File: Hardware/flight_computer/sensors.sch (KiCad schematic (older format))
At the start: 21 parts

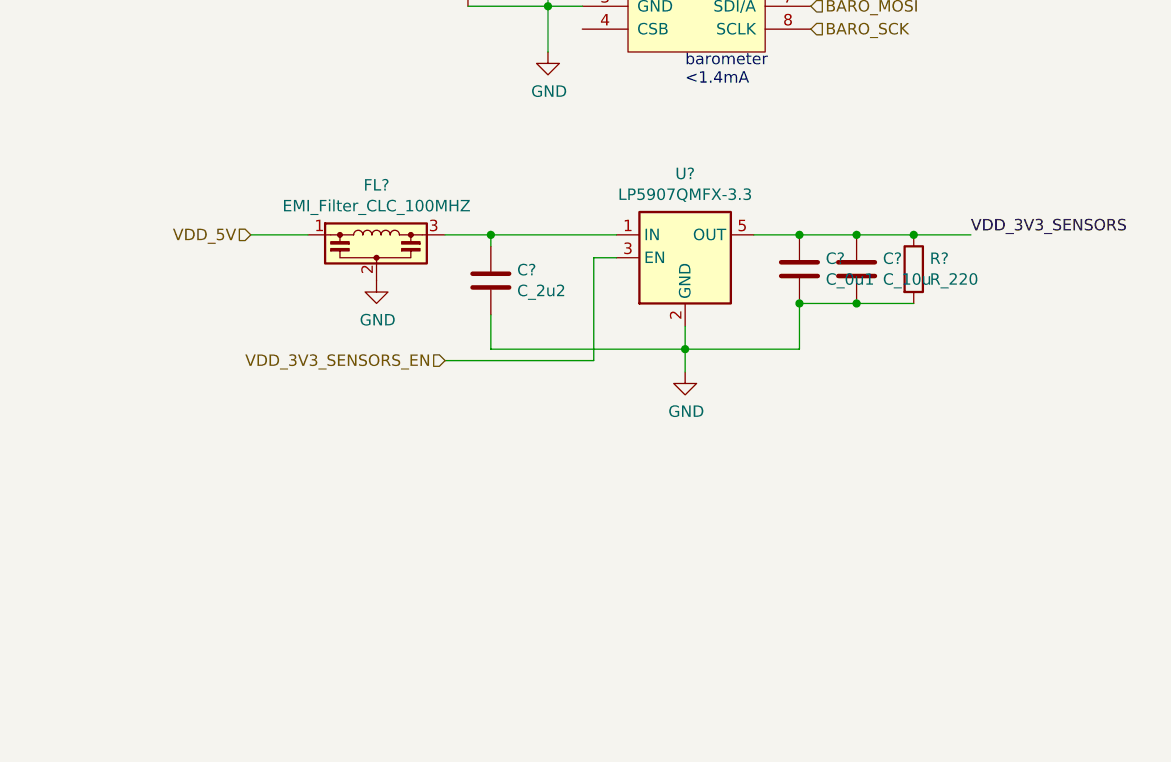
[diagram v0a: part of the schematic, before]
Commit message: added components, rerranged things to slow down dan
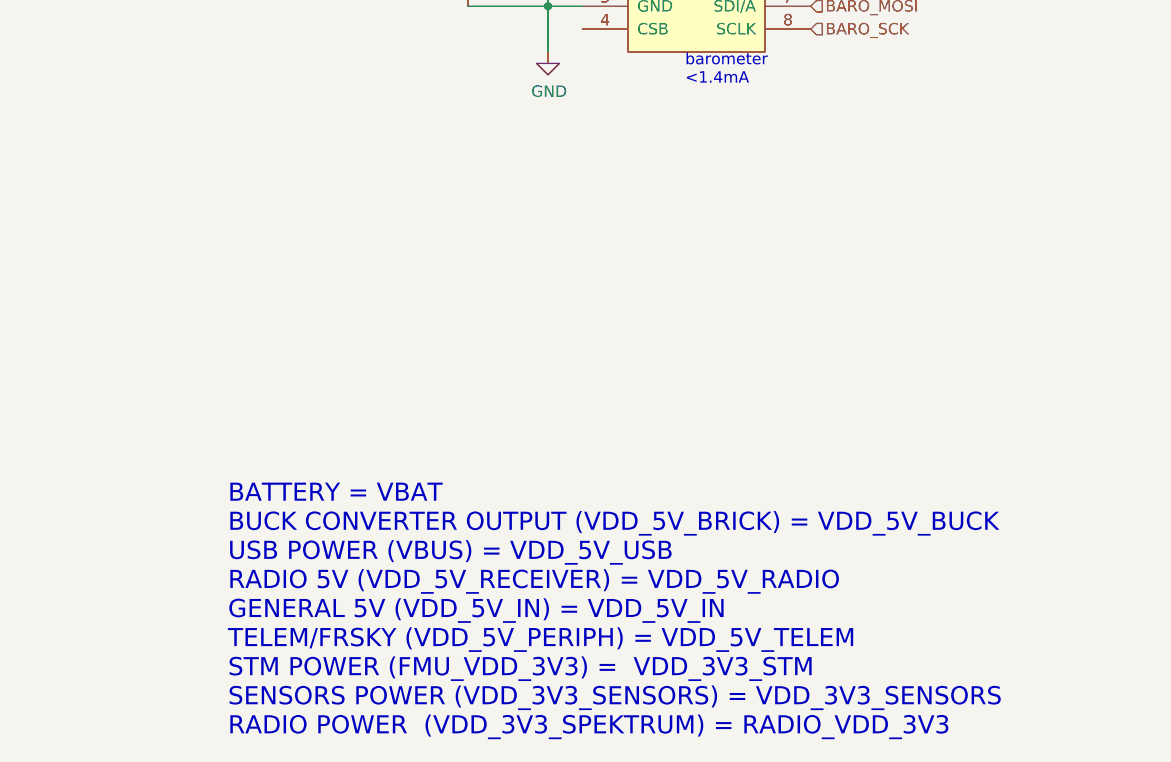
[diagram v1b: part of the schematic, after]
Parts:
- removed C?: C_10u, Capacitors_SMD:C_0805, symbol openDrone_parts:C_10u
- removed C?: C_0u1, Capacitors_SMD:C_0805, symbol openDrone_parts:C_0u1
- removed C?: C_2u2, Capacitors_SMD:C_0805, symbol openDrone_parts:C_2u2
- removed FL?: EMI_Filter_CLC_100MHZ, drone_footprints:NFL21SP107X1C3D, symbol openDrone_parts:EMI_Filter_CLC_100MHZ
- removed R?: R_220, Resistors_SMD:R_0805, symbol openDrone_parts:R_220
- removed U?: LP5907QMFX-3.3, TO_SOT_Packages_SMD:SOT-23-5, symbol openDrone_parts:LP5907QMFX-3.3
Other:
- note added: "BATTERY = VBAT\nBUCK CONVERTER OUTPUT (VDD_5V_BRICK) = VDD_5V_BUCK\nUSB POWER (VBUS) = VDD_5V_USB\nRADIO 5V (VDD_5V_RECEIVER) = VDD_5V_RADIO\nGENERAL 5V (VDD_5V_IN) = VDD_5V_IN\nTELEM/FRSKY (VDD_5V_PERIPH) = VDD_5V_TELEM\nSTM POWER (FMU_VDD_3V3) = VDD_3V3_STM\nSENSORS POWER (VDD_3V3_SENSORS) = VDD_3V3_SENSORS\nRADIO POWER (VDD_3V3_SPEKTRUM) = RADIO_VDD_3V3\n"
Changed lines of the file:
@@
 $Descr A4 11693 8268
 encoding utf-8
-Sheet 2 4
+Sheet 2 5
 Title ""
 Date ""
@@
 Wire Wire Line
 	8600 2850 8200 2850
-$Comp
-L openDrone_parts:LP5907QMFX-3.3 U?
-U 1 1 5F953D79
-P 9150 4250
-F 0 "U?" H 9150 4617 50  0000 C CNN
-F 1 "LP5907QMFX-3.3" H 9150 4526 50  0000 C CNN
-F 2 "TO_SOT_Packages_SMD:SOT-23-5" H 9150 4600 50  0001 C CNN
-F 3 "http://www.ti.com/lit/ds/symlink/lp5907.pdf" H 9150 4750 50  0001 C CNN
-F 4 "296-40365-1-ND" H 9200 4650 50  0001 C CNN "DPN"
-F 5 "LP5907QMFX-3.3Q1" H 9100 4750 50  0001 C CNN "MPN"
-	1    9150 4250
-	1    0    0    -1
-$EndComp
-$Comp
-L openDrone_parts:R_220 R?
-U 1 1 5F954E14
-P 10150 4300
-F 0 "R?" V 10104 4370 50  0000 L CNN
-F 1 "R_220" V 10195 4370 50  0000 L CNN
-F 2 "Resistors_SMD:R_0805" H 9350 4450 50  0001 C CNN
-F 3 "" H 9850 4800 50  0001 C CNN
-F 4 "311-220CRCT-ND" H 9500 4550 60  0001 C CNN "DPN"
-	1    10150 4300
-	0    1    1    0
-$EndComp
-$Comp
-L openDrone_parts:C_10u C?
-U 1 1 5F9559A3
-P 9900 4300
-F 0 "C?" H 10015 4346 50  0000 L CNN
-F 1 "C_10u" H 10015 4255 50  0000 L CNN
-F 2 "Capacitors_SMD:C_0805" H 9938 4150 50  0001 C CNN
-F 3 "" H 9925 4400 50  0001 C CNN
-F 4 "490-16824-1-ND" H 9900 4300 60  0001 C CNN "DPN"
-	1    9900 4300
-	1    0    0    -1
-$EndComp
-$Comp
-L openDrone_parts:C_0u1 C?
-U 1 1 5F956265
-P 9650 4300
-F 0 "C?" H 9765 4346 50  0000 L CNN
-F 1 "C_0u1" H 9765 4255 50  0000 L CNN
-F 2 "Capacitors_SMD:C_0805" H 9688 4150 50  0001 C CNN
-F 3 "https://www.digikey.com/product-detail/en/kemet/C0805C104Z4VACTU/399-9159-1-ND/3522677" H 9675 4400 50  0001 C CNN
-F 4 "478-3352-1-ND" H 9650 4300 60  0001 C CNN "DPN"
-	1    9650 4300
-	1    0    0    -1
-$EndComp
-$Comp
-L openDrone_parts:C_2u2 C?
-U 1 1 5F956971
-P 8300 4350
-F 0 "C?" H 8415 4396 50  0000 L CNN
-F 1 "C_2u2" H 8415 4305 50  0000 L CNN
-F 2 "Capacitors_SMD:C_0805" H 8338 4200 50  0001 C CNN
-F 3 "" H 8325 4450 50  0001 C CNN
-F 4 "445-13254-1-ND" H 8300 4350 60  0001 C CNN "DPN"
-	1    8300 4350
-	1    0    0    -1
-$EndComp
-Text HLabel 8100 4700 0    50   Input ~ 0
-VDD_3V3_SENSORS_EN
-$Comp
-L power:GND #PWR?
-U 1 1 5F9574AD
-P 9150 4750
-F 0 "#PWR?" H 9150 4500 50  0001 C CNN
-F 1 "GND" H 9155 4577 50  0000 C CNN
-F 2 "" H 9150 4750 50  0001 C CNN
-F 3 "" H 9150 4750 50  0001 C CNN
-	1    9150 4750
-	1    0    0    -1
-$EndComp
-Wire Wire Line
-	9450 4150 9650 4150
-Connection ~ 9650 4150
-Wire Wire Line
-	9650 4150 9900 4150
-Connection ~ 9900 4150
-Wire Wire Line
-	9900 4150 10150 4150
-Connection ~ 10150 4150
-Wire Wire Line
-	10150 4150 10400 4150
-Wire Wire Line
-	10150 4450 9900 4450
-Wire Wire Line
-	9900 4450 9650 4450
-Connection ~ 9900 4450
-Wire Wire Line
-	9650 4450 9650 4650
-Wire Wire Line
-	9650 4650 9150 4650
-Wire Wire Line
-	8300 4650 8300 4500
-Connection ~ 9650 4450
-Wire Wire Line
-	8850 4150 8300 4150
-Wire Wire Line
-	8300 4150 8300 4200
-Wire Wire Line
-	8100 4700 8750 4700
-Wire Wire Line
-	8750 4700 8750 4250
-Wire Wire Line
-	8750 4250 8850 4250
-Wire Wire Line
-	9150 4550 9150 4650
-Connection ~ 9150 4650
-Wire Wire Line
-	9150 4650 8300 4650
-Wire Wire Line
-	9150 4650 9150 4750
-Text HLabel 7250 4150 0    50   Input ~ 0
-VDD_5V
 Text Label 2700 2450 2    50   ~ 0
 VDD_3V3_SENSORS
@@
 VDD_3V3_SENSORS
 Text Label 8200 2850 2    50   ~ 0
-VDD_3V3_SENSORS
-Text Label 10400 4150 0    50   ~ 0
 VDD_3V3_SENSORS
 $Comp
@@
 Text Notes 3100 4000 0    50   ~ 0
 Note for the EMI filter \nthat the GPS here is at 3.3V \nnot 5V like in the pixracer
-$Comp
-L openDrone_parts:EMI_Filter_CLC_100MHZ FL?
-U 1 1 5FA22B48
-P 7800 4250
-F 0 "FL?" H 7800 4567 50  0000 C CNN
-F 1 "EMI_Filter_CLC_100MHZ" H 7800 4476 50  0000 C CNN
-F 2 "drone_footprints:NFL21SP107X1C3D" H 8450 4750 50  0001 C CNN
-F 3 "" V 7800 4250 50  0001 C CNN
-F 4 "490-2540-1-ND" H 8700 4500 50  0001 C CNN "DPN"
-F 5 "NFL21SP107X1C3D" H 8450 4600 50  0001 C CNN "MPN"
-	1    7800 4250
-	1    0    0    -1
-$EndComp
-Wire Wire Line
-	8300 4150 8100 4150
-Connection ~ 8300 4150
-$Comp
-L power:GND #PWR?
-U 1 1 5FA26F34
-P 7800 4350
-F 0 "#PWR?" H 7800 4100 50  0001 C CNN
-F 1 "GND" H 7805 4177 50  0000 C CNN
-F 2 "" H 7800 4350 50  0001 C CNN
-F 3 "" H 7800 4350 50  0001 C CNN
-	1    7800 4350
-	1    0    0    -1
-$EndComp
-Wire Wire Line
-	7250 4150 7500 4150
+Text Notes 7150 6350 0    79   ~ 0
+BATTERY = VBAT\nBUCK CONVERTER OUTPUT (VDD_5V_BRICK) = VDD_5V_BUCK\nUSB POWER (VBUS) = VDD_5V_USB\nRADIO 5V (VDD_5V_RECEIVER) = VDD_5V_RADIO\nGENERAL 5V (VDD_5V_IN) = VDD_5V_IN\nTELEM/FRSKY (VDD_5V_PERIPH) = VDD_5V_TELEM\nSTM POWER (FMU_VDD_3V3) =  VDD_3V3_STM\nSENSORS POWER (VDD_3V3_SENSORS) = VDD_3V3_SENSORS\nRADIO POWER  (VDD_3V3_SPEKTRUM) = RADIO_VDD_3V3\n
 $EndSCHEMATC
